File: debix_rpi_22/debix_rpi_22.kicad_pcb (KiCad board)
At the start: 2 copper layers, 2 parts, among them J1 Conn_01x24, J3 RPi 22 Pin MIPI CSI-2

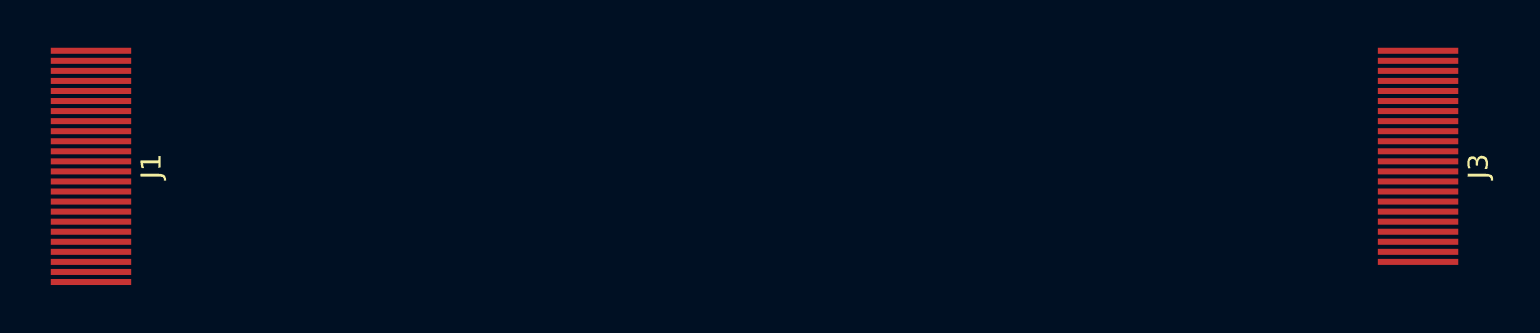
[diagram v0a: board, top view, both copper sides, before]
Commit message: just the lanes.
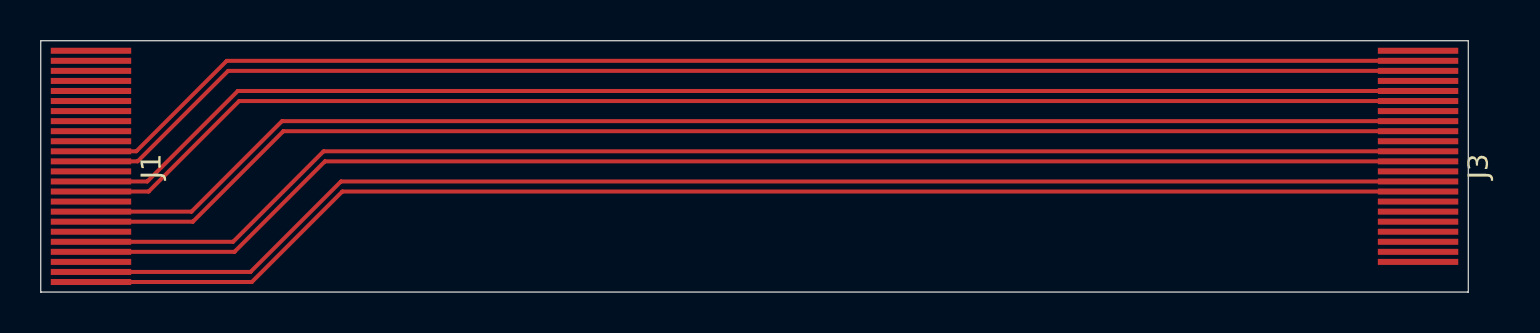
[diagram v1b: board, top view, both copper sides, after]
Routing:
- net /csi_d3_P: track 0.00 -> 67.9 mm
- net /csi_d3_N: track 0.00 -> 67.9 mm
- net /csi_d2_P: track 0.00 -> 67.9 mm
- net /csi_d2_N: track 0.00 -> 67.9 mm
- net /csi_d1_P: track 0.00 -> 67.9 mm
- net /csi_d1_N: track 0.00 -> 67.9 mm
- net /csi_d0_P: track 0.00 -> 67.9 mm
- net /csi_d0_N: track 0.00 -> 67.9 mm
- net /csi_clk_P: track 0.00 -> 67.9 mm
- net /csi_clk_N: track 0.00 -> 67.9 mm
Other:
- board outline added: 71 x 12.5 mm
